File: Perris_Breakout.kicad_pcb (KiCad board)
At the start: 2 copper layers, 67.3 x 67.3 mm, 21 parts, among them J1 PERRI_1, J10 SDA, J11 GND, J12 GND, J13 SCL, J14 SCL, J2 PERRI_2, J3 PERRI_3, J4 PERRI_4, J5 PERRI_5, J6 PERRI_6, J7 PERRI_7, J8 PERRI_8, J9 SDA

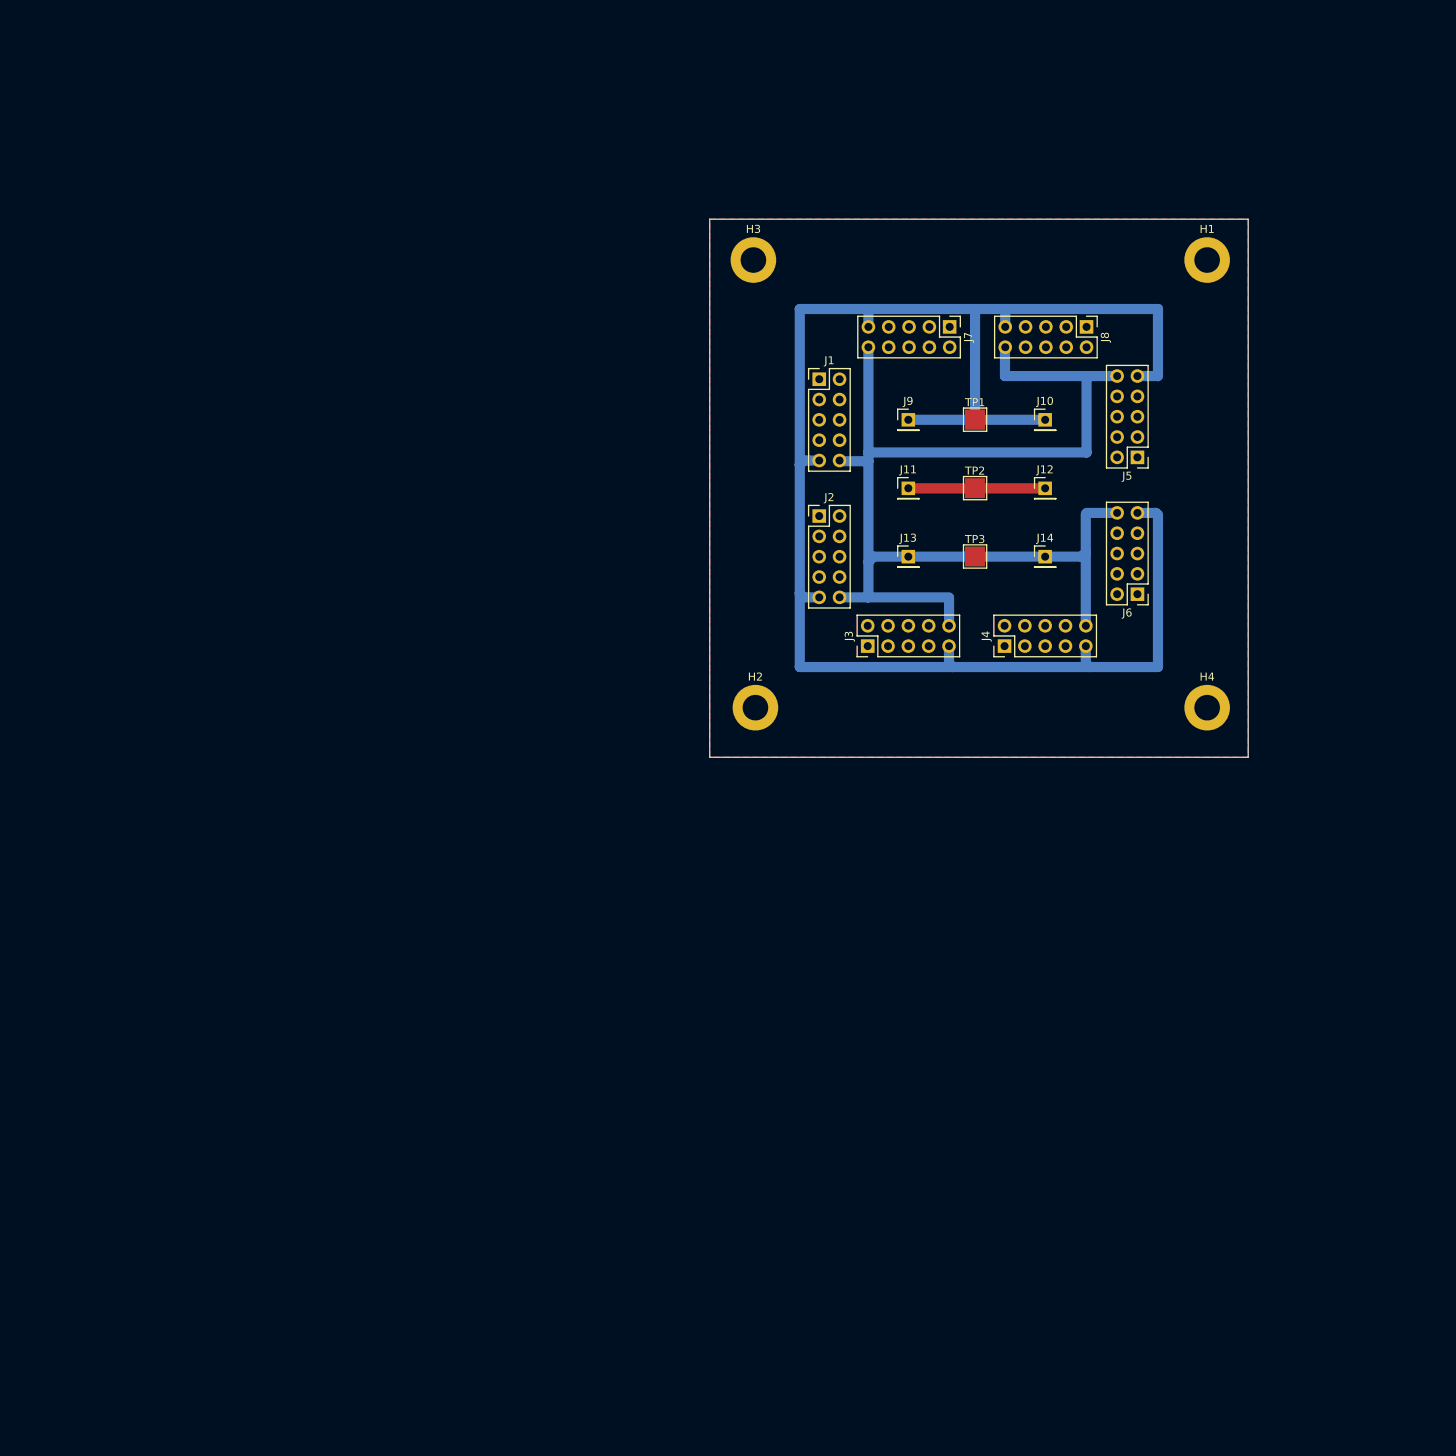
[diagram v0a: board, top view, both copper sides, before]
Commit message: More Perris
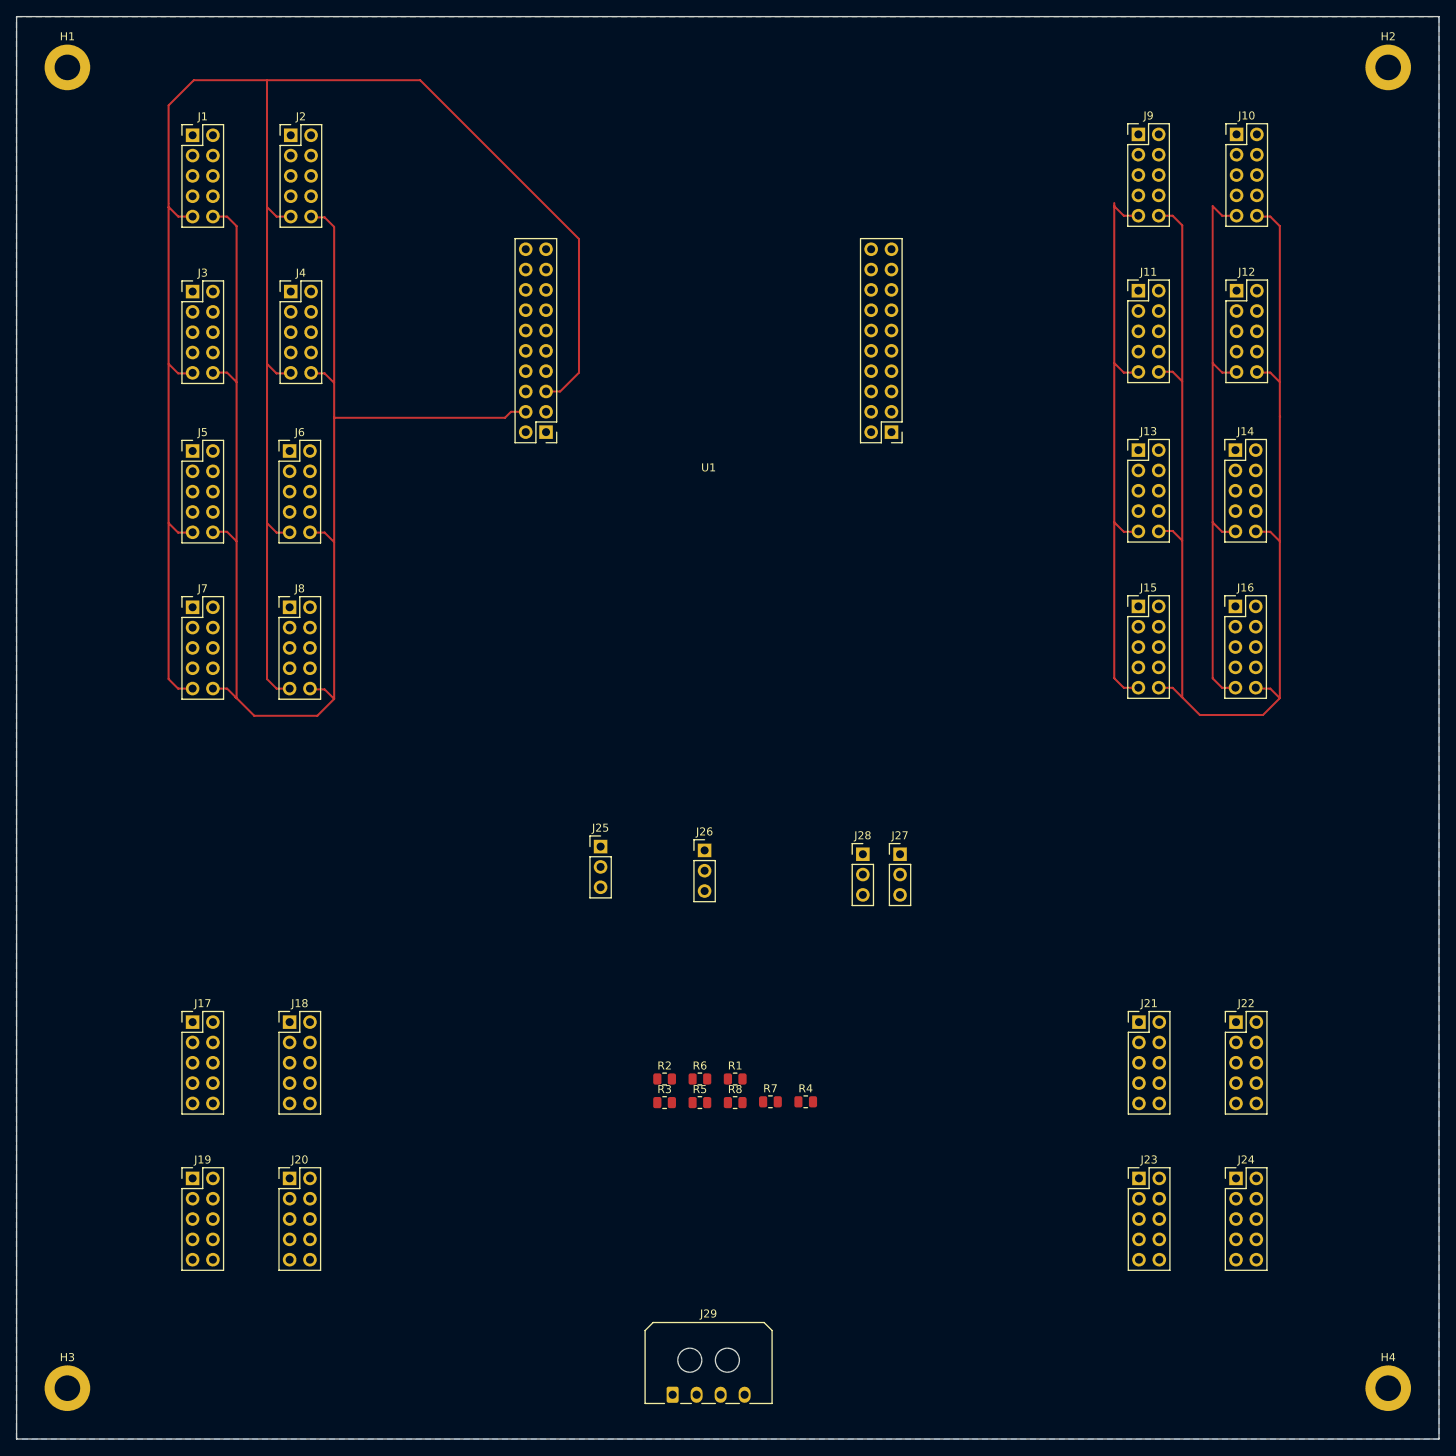
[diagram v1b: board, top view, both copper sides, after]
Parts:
- removed TP1: SDA, TestPoint:TestPoint_Pad_2.5x2.5mm
- removed TP2: GND, TestPoint:TestPoint_Pad_2.5x2.5mm
- removed TP3: SCL, TestPoint:TestPoint_Pad_2.5x2.5mm
- added J15: PERRI_15, HELIX:Perri_conn_2x5_Reverse, F.Cu at (140.2, 86.4)
- added J16: PERRI_16, HELIX:Perri_conn_2x5_Reverse, F.Cu at (152.4, 86.4)
- added J17: PERRI_17, HELIX:Perri_conn_2x5_Reverse, F.Cu at (22.0, 138.4)
- added J18: PERRI_18, HELIX:Perri_conn_2x5_Reverse, F.Cu at (34.1, 138.4)
- added J19: PERRI_19, HELIX:Perri_conn_2x5_Reverse, F.Cu at (22.0, 157.9)
- added J20: PERRI_20, HELIX:Perri_conn_2x5_Reverse, F.Cu at (34.1, 157.9)
- added J21: PERRI_21, HELIX:Perri_conn_2x5_Reverse, F.Cu at (140.3, 138.4)
- added J22: PERRI_22, HELIX:Perri_conn_2x5_Reverse, F.Cu at (152.4, 138.4)
- added J23: PERRI_23, HELIX:Perri_conn_2x5_Reverse, F.Cu at (140.3, 157.9)
- added J24: PERRI_24, HELIX:Perri_conn_2x5_Reverse, F.Cu at (152.4, 157.9)
- added J25: Probe 0, Connector_PinHeader_2.54mm:PinHeader_1x03_P2.54mm_Vertical, F.Cu at (73.0, 116.5)
- added J26: Probe 1, Connector_PinHeader_2.54mm:PinHeader_1x03_P2.54mm_Vertical, F.Cu at (86.0, 116.9)
- added J27: Probe 2, Connector_PinHeader_2.54mm:PinHeader_1x03_P2.54mm_Vertical, F.Cu at (110.4, 117.4)
- added J28: Probe 3, Connector_PinHeader_2.54mm:PinHeader_1x03_P2.54mm_Vertical, F.Cu at (105.8, 117.4)
- added J29: Power, Connector_Molex:Molex_Micro-Fit_3.0_43650-0400_1x04_P3.00mm_Horizontal, F.Cu at (82.0, 185.0)
- added R1: Resistor, Resistor_SMD:R_0805_2012Metric, F.Cu at (89.8, 145.5)
- added R2: Resistor, Resistor_SMD:R_0805_2012Metric, F.Cu at (81.0, 145.5)
- added R3: Resistor, Resistor_SMD:R_0805_2012Metric, F.Cu at (81.0, 148.4)
- added R4: Resistor, Resistor_SMD:R_0805_2012Metric, F.Cu at (98.6, 148.3)
- added R5: Resistor, Resistor_SMD:R_0805_2012Metric, F.Cu at (85.4, 148.4)
- added R6: Resistor, Resistor_SMD:R_0805_2012Metric, F.Cu at (85.4, 145.5)
- added R7: Resistor, Resistor_SMD:R_0805_2012Metric, F.Cu at (94.2, 148.3)
- added R8: Resistor, Resistor_SMD:R_0805_2012Metric, F.Cu at (89.8, 148.4)
- added U1: EK-TM4C123GXL, HELIX:TM4C123GXL_launchpad_male_connector, F.Cu at (86.5, 53.2)
- H1, H2, H3, H4: value MountingHole_Pad -> Mount
- J10: value SDA -> PERRI_10; footprint Connector_PinHeader_2.54mm:PinHeader_1x01_P2.54mm_Vertical -> HELIX:Perri_conn_2x5_Reverse
- J11: value GND -> PERRI_11; footprint Connector_PinHeader_2.54mm:PinHeader_1x01_P2.54mm_Vertical -> HELIX:Perri_conn_2x5_Reverse
- J12: value GND -> PERRI_12; footprint Connector_PinHeader_2.54mm:PinHeader_1x01_P2.54mm_Vertical -> HELIX:Perri_conn_2x5_Reverse
- J13: value SCL -> PERRI_13; footprint Connector_PinHeader_2.54mm:PinHeader_1x01_P2.54mm_Vertical -> HELIX:Perri_conn_2x5_Reverse
- J14: value SCL -> PERRI_14; footprint Connector_PinHeader_2.54mm:PinHeader_1x01_P2.54mm_Vertical -> HELIX:Perri_conn_2x5_Reverse
- J9: value SDA -> PERRI_9; footprint Connector_PinHeader_2.54mm:PinHeader_1x01_P2.54mm_Vertical -> HELIX:Perri_conn_2x5_Reverse
- moved H3 165.0 mm to (6.35, 184.2)
- moved H1 144.5 mm to (6.35, 19.1)
- moved J5 118.1 mm to (22.0, 67.0), turned to 0 degrees
- moved H2 112.5 mm to (171.4, 19.1)
- moved J6 107.5 mm to (34.1, 67.0), turned to 0 degrees
- moved J8 105.6 mm to (34.1, 86.5), turned to 0 degrees
- moved J7 100.9 mm to (22.0, 86.5), turned to 0 degrees
- moved J4 99.6 mm to (34.3, 47.1), turned to 0 degrees
- moved J3 95.3 mm to (22.0, 47.1), turned to 0 degrees
- moved H4 88.0 mm to (171.4, 184.2)
- moved J1 84.1 mm to (22.0, 27.5)
- moved J2 81.4 mm to (34.3, 27.5)
- moved J9 45.8 mm to (140.2, 27.4)
- moved J10 43.0 mm to (152.5, 27.4)
- moved J11 37.9 mm to (140.2, 47.0)
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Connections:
- H1 pad 1: /GND -> GND
- H2 pad 1: /GND -> GND
- H3 pad 1: /GND -> GND
- H4 pad 1: /GND -> GND
- J1 pad 10: /GND -> GND
- J1 pad 5: /SCL -> /SCL_0
- J1 pad 6: /SDA -> /SDA_0
- J10 pad 1: /SDA -> unconnected-(J10-Pad1)
- J11 pad 1: /GND -> unconnected-(J11-Pad1)
- J12 pad 1: /GND -> unconnected-(J12-Pad1)
- J13 pad 1: /SCL -> unconnected-(J13-Pad1)
- J14 pad 1: /SCL -> unconnected-(J14-Pad1)
- J2 pad 10: /GND -> GND
- J2 pad 5: /SCL -> /SCL_0
- J2 pad 6: /SDA -> /SDA_0
- J3 pad 10: /GND -> GND
- J3 pad 5: /SCL -> /SCL_0
- J3 pad 6: /SDA -> /SDA_0
- J4 pad 10: /GND -> GND
- J4 pad 5: /SCL -> /SCL_0
- J4 pad 6: /SDA -> /SDA_0
- J5 pad 10: /GND -> GND
- J5 pad 5: /SCL -> /SCL_0
- J5 pad 6: /SDA -> /SDA_0
- J6 pad 10: /GND -> GND
- J6 pad 5: /SCL -> /SCL_0
- J6 pad 6: /SDA -> /SDA_0
- J7 pad 10: /GND -> GND
- J7 pad 5: /SCL -> /SCL_0
- J7 pad 6: /SDA -> /SDA_0
- J8 pad 10: /GND -> GND
- J8 pad 5: /SCL -> /SCL_0
- J8 pad 6: /SDA -> /SDA_0
- J9 pad 1: /SDA -> unconnected-(J9-Pad1)
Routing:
- net /SDA_0: track 0.00 -> 257.2 mm
- net /SDA: track 213.1 -> 0.00 mm
- net /SCL_0: track 0.00 -> 184.4 mm
- net /SCL_1: track 0.00 -> 160.2 mm
- net /SCL: track 152.0 -> 0.00 mm
- net /SDA_1: track 0.00 -> 146.4 mm
- net /GND: track 17.1 -> 0.00 mm
- added copper zone on B.Cu, net GND
- removed copper zone on F.Cu, net /GND
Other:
- board size 67.3 x 67.3 mm -> 177.8 x 177.8 mm
